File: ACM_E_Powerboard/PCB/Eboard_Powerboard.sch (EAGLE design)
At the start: 21 parts, among them IC1 TCMD4000, Q1 NGD8201ANT4G, Q2 NGD8201ANT4G, Q3 NGD8201ANT4G

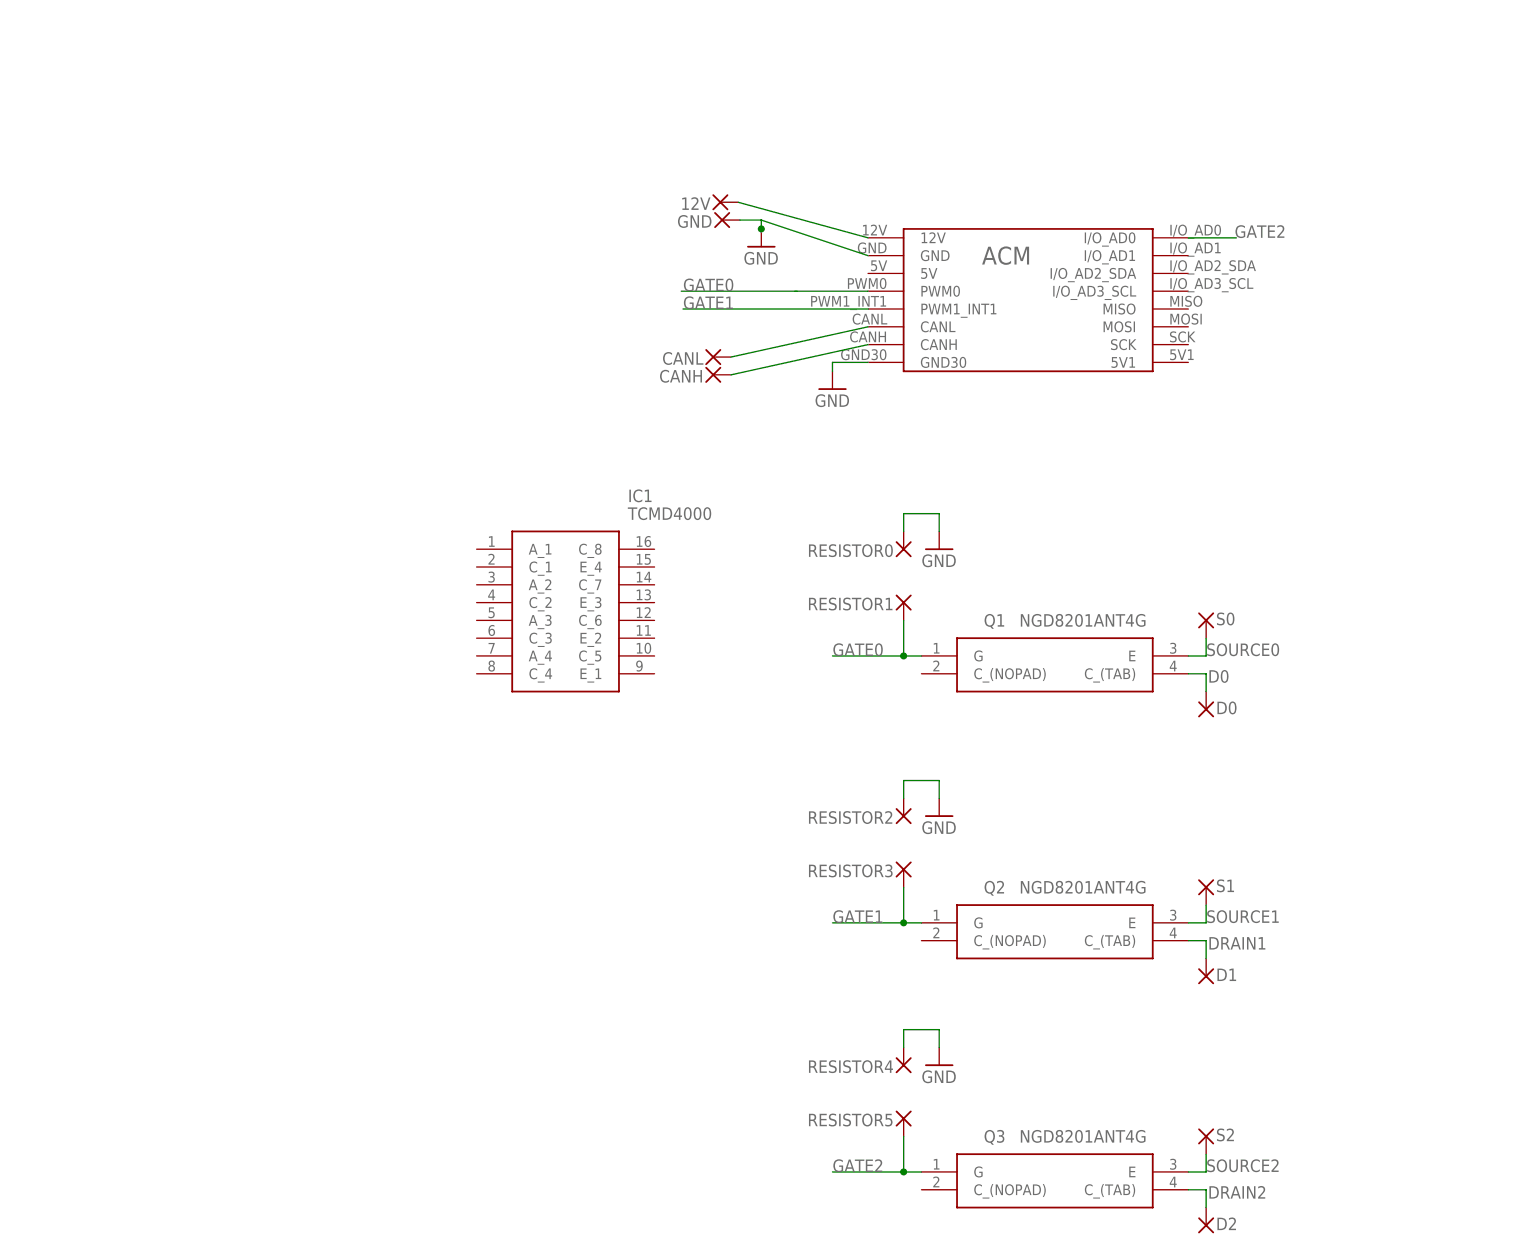
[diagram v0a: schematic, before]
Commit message: Powerboard RDY
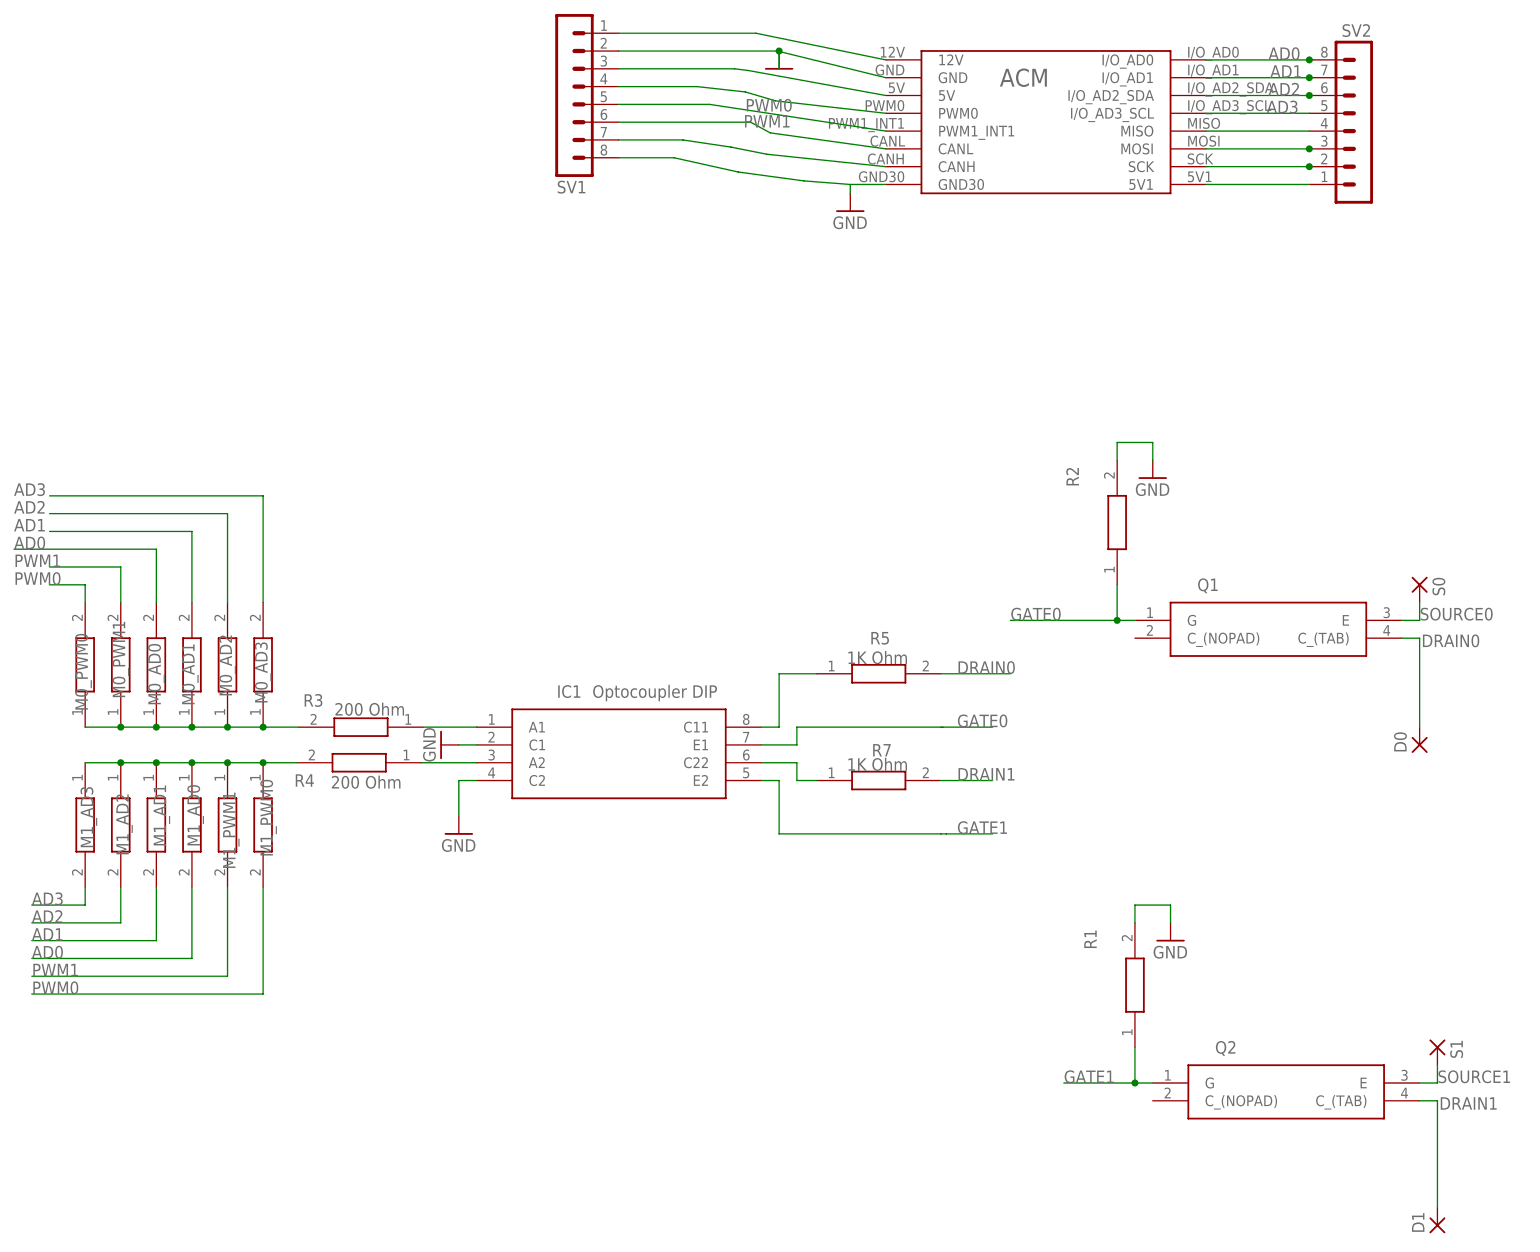
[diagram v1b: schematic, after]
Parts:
- removed 12V, CANH, CANL, GND, RESISTOR0, RESISTOR1, RESISTOR2, RESISTOR3, RESISTOR4, RESISTOR5: (no value), wirepad:2,15/1,0
- removed D2, S2: (no value), wirepad:2,54/1,0
- removed Q3: NGD8201ANT4G, NGD8201ANT4G_Mosfet:NGD8201ANT4G
- added M0_AD0, M0_AD1, M0_AD2, M0_AD3, M0_PWM0, M0_PWM1, M1_AD0, M1_AD1, M1_AD2, M1_AD3, M1_PWM0, M1_PWM1, R1, R2: ERA-3AEB2262V, ERA-3AEB2262V(0603 Resistor):ERA-3AEB2262V
- added R3, R4: 200 Ohm, ERA-3AEB2262V(0603 Resistor):ERA-3AEB2262V
- added R5, R7: 1K Ohm, ERA-3AEB2262V(0603 Resistor):ERA-3AEB2262V
- added SV1, SV2: (no value), con-lstb:MA08-1W
- D0, D1, S0, S1: value (none) -> WIREPADSMD5-2,5; device wirepad:2,54/1,0 -> wirepad:WIREPADSMD5-2,5
- IC1: value TCMD4000 -> Optocoupler DIP; device SFH6916:TCMD4000 -> TLP350(F):TLP350(F)
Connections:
- removed net D0: D0.P, Q1.C_(TAB)
- removed net DRAIN2: D2.P, Q3.C_(TAB)
- removed net GATE2: Q3.G, RESISTOR5.P, U$1.I/O_AD0
- removed net SOURCE2: Q3.E, S2.P
- new net AD0: M0_AD0.2, M1_AD0.2, SV2.8, U$1.I/O_AD0
- new net AD1: M0_AD1.2, M1_AD1.2, SV2.7, U$1.I/O_AD1
- new net AD2: M0_AD2.2, M1_AD2.2, SV2.6, U$1.I/O_AD2_SDA
- new net AD3: M0_AD3.2, M1_AD3.2, SV2.5, U$1.I/O_AD3_SCL
- new net DRAIN0: D0.P, Q1.C_(TAB), R5.2
- new net N$1: SV1.3, U$1.5V
- new net N$10: SV2.3, U$1.MOSI
- new net N$11: SV2.2, U$1.SCK
- new net N$12: SV2.1, U$1.5V1
- new net N$13: IC1.C22, R7.1
- new net N$15: M0_AD0.1, M0_AD1.1, M0_AD2.1, M0_AD3.1, M0_PWM0.1, M0_PWM1.1, R3.2
- new net N$16: M1_AD0.1, M1_AD1.1, M1_AD2.1, M1_AD3.1, M1_PWM0.1, M1_PWM1.1, R4.2
- new net N$2: IC1.A1, R3.1
- new net N$6: IC1.A2, R4.1
- new net N$7: IC1.C11, R5.1
- new net N$9: SV2.4, U$1.MISO
- new net PWM0: M0_PWM0.2, M1_PWM0.2, SV1.4, U$1.PWM0
- new net PWM1: M0_PWM1.2, M1_PWM1.2, SV1.5, U$1.PWM1_INT1
- net DRAIN1: now also R7.2
- net GATE0: now also IC1.E1, R2.1; no longer RESISTOR1.P, U$1.PWM0
- net GATE1: now also IC1.E2, R1.1; no longer RESISTOR3.P, U$1.PWM1_INT1
- net GND: now also IC1.C1, IC1.C2, R1.2, R2.2, SV1.2, SV1.8; no longer GND.P, RESISTOR0.P, RESISTOR2.P, RESISTOR4.P
- net N$3: now also SV1.1; no longer 12V.P
- net N$4: now also SV1.6; no longer CANL.P
- net N$5: now also SV1.7; no longer CANH.P
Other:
- moved on the sheet: Q1, Q2
